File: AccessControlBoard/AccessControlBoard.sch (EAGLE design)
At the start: 9 parts, among them J1 4p-2.54, X1 1751248

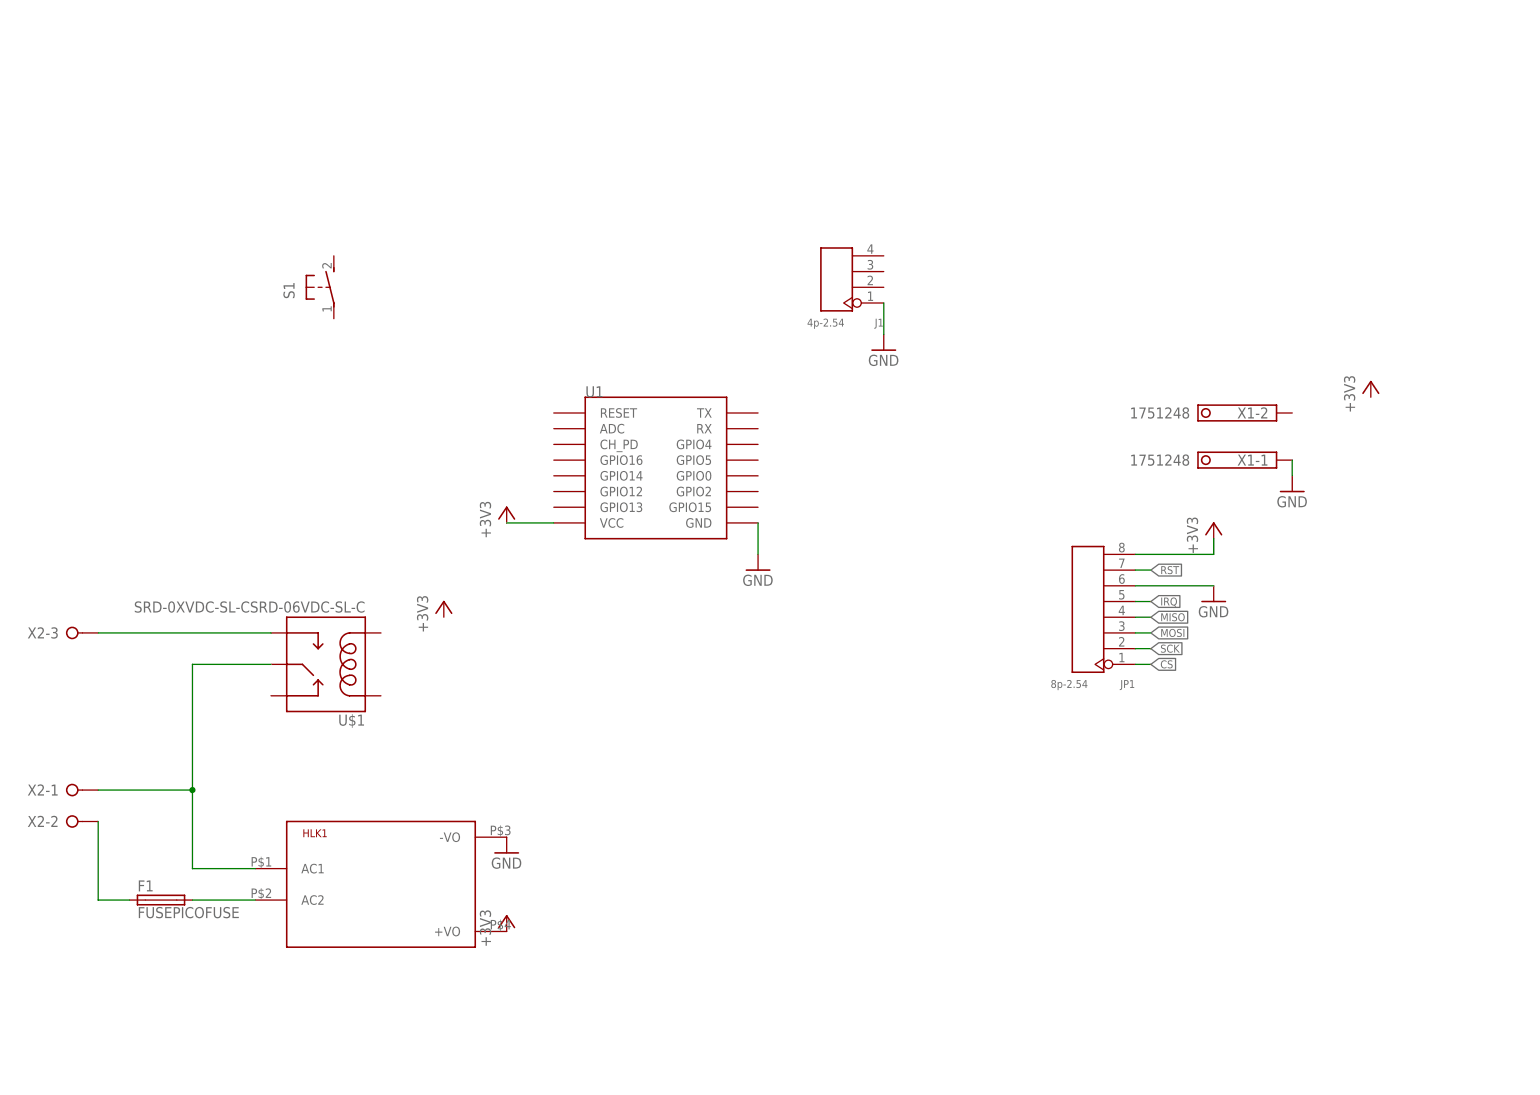
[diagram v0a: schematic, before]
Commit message: update
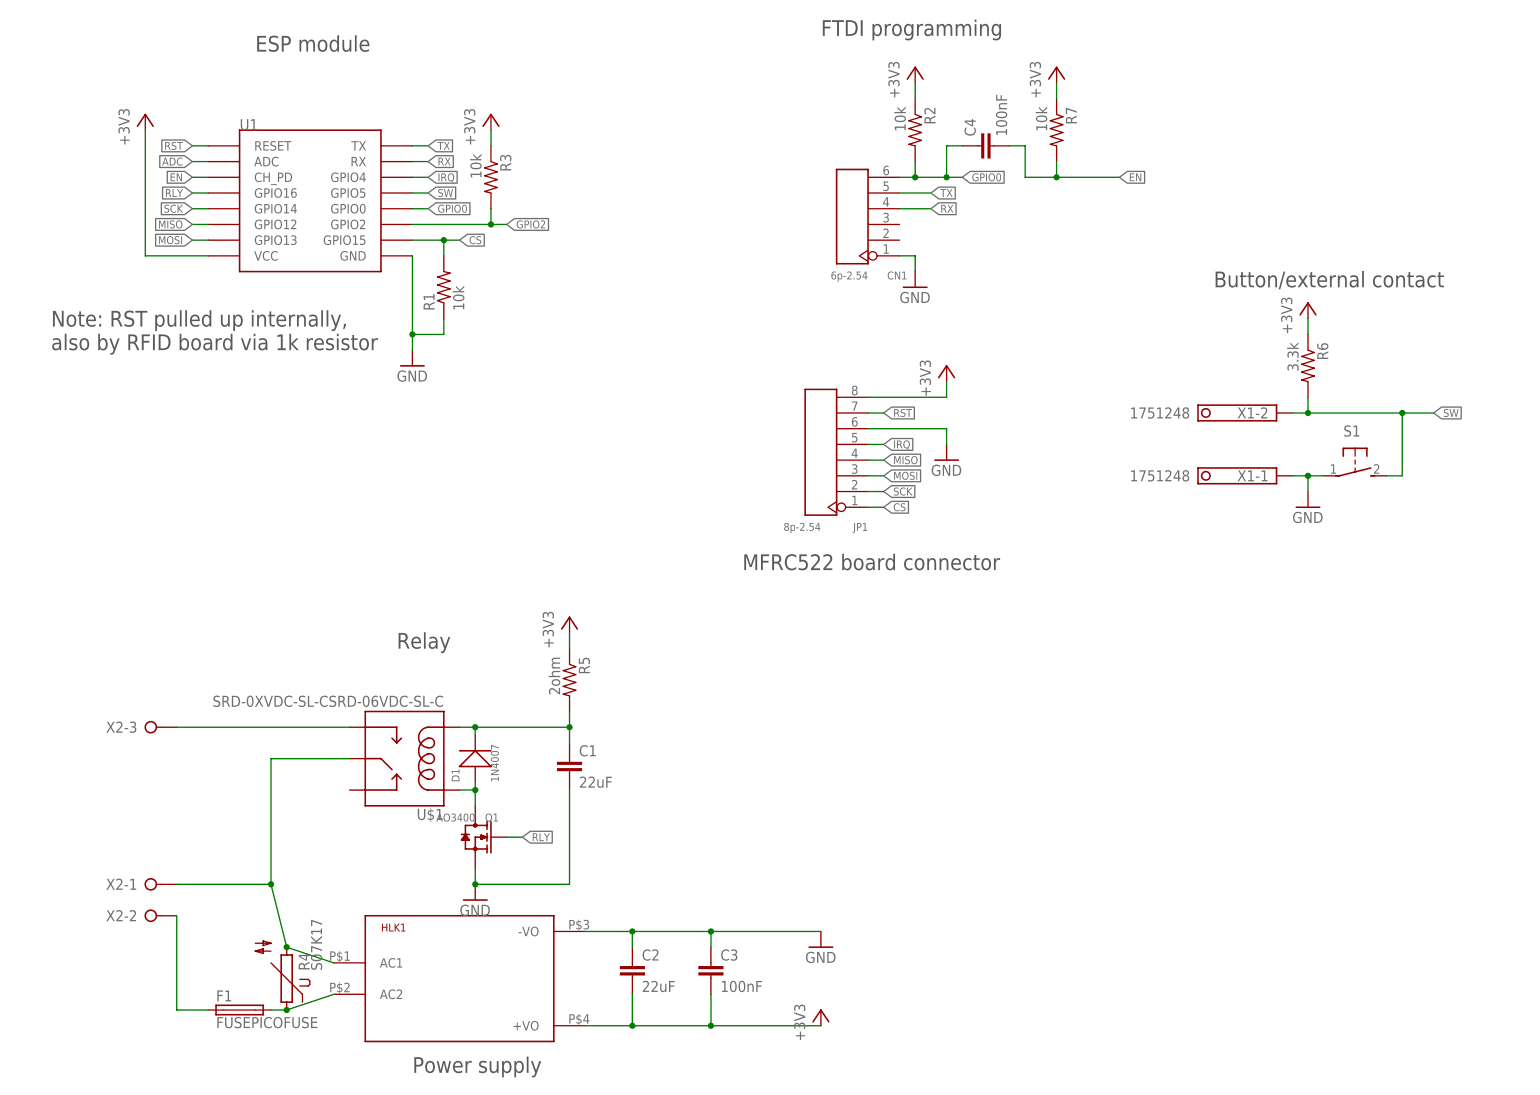
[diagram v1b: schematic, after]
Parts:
- removed J1: 4p-2.54, Seeed-Connector:DIP-BLACK-FEMALE-HEADER-VERT(4P-2.54)
- added C1, C2: 22uF, rcl:C-EUC0805K
- added C3, C4: 100nF, rcl:C-EUC0603K
- added CN1: 6p-2.54, Seeed-Connector:DIP-BLACK-FEMALE-HEADER-VERT(6P-2.54)
- added D1: 1N4007, Seeed-Diode:DIODE-GEN-PURPOSE-1KV-1A(DO-214AC)
- added Q1: AO3400, Seeed-Transistor:SMD-MOSFET-N-CH-60V-300MA-LOGIC-LEVEL-FET-2N7002(SOT-23)
- added R1, R2, R3, R7: 10k, resistor:R-US_R0603
- added R4: S07K17, varistor:S07K17
- added R5: 2ohm, resistor:R-US_R0603
- added R6: 3.3k, resistor:R-US_R0603
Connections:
- new net ADC: U1.ADC
- new net EN: C4.2, R7.2, U1.CH_PD
- new net GPIO0: C4.1, CN1.6, R2.2, U1.GPIO0
- new net GPIO2: R3.2, U1.GPIO2
- new net N$5: C1.1, D1.-, R5.2, U$1.COIL0
- new net N$8: D1.+, Q1.D, U$1.COIL1
- new net RLY: Q1.G, U1.GPIO16
- new net RX: CN1.4, U1.RX
- new net SW: R6.2, S1.S, U1.GPIO5, X1-2.K
- new net TX: CN1.5, U1.TX
- net +3V3: now also C2.2, C3.2, R2.1, R3.1, R5.1, R6.1, R7.1
- net CS: now also R1.2, U1.GPIO15
- net GND: now also C1.2, C2.1, C3.1, CN1.1, Q1.S, R1.1, S1.P; no longer J1.P$1
- net IRQ: now also U1.GPIO4
- net MISO: now also U1.GPIO12
- net MOSI: now also U1.GPIO13
- net N$2: now also R4.2
- net N$3: now also R4.1
- net RST: now also U1.RESET
- net SCK: now also U1.GPIO14
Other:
- note added: "Button/external contact"
- note added: "ESP module"
- note added: "FTDI programming"
- note added: "MFRC522 board connector"
- note added: "Note: RST pulled up internally, also by RFID board via 1k resistor"
- note added: "Power supply"
- note added: "Relay"
- moved on the sheet: F1, HLK1, JP1, S1, U$1, U1, X1-1, X2-1, X2-2, X2-3
